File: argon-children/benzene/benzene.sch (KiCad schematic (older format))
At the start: 9 parts, among them U1 Conn1, U2 SPI FLASH, U3 Conn2

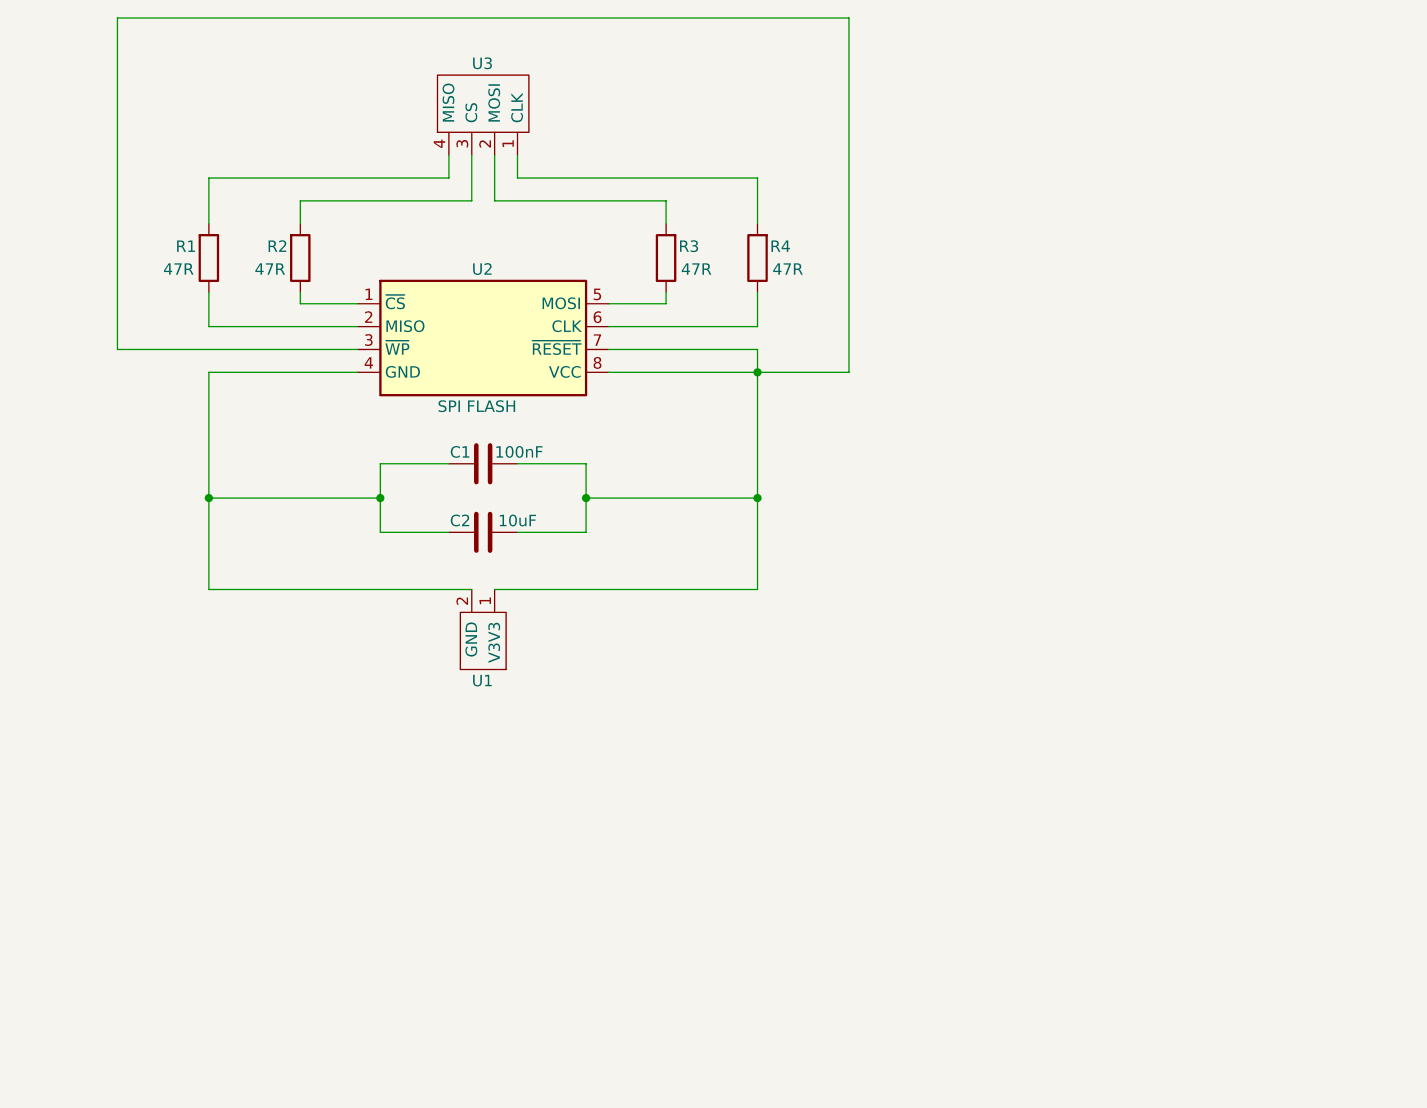
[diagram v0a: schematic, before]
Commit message: Add 555 to benzene
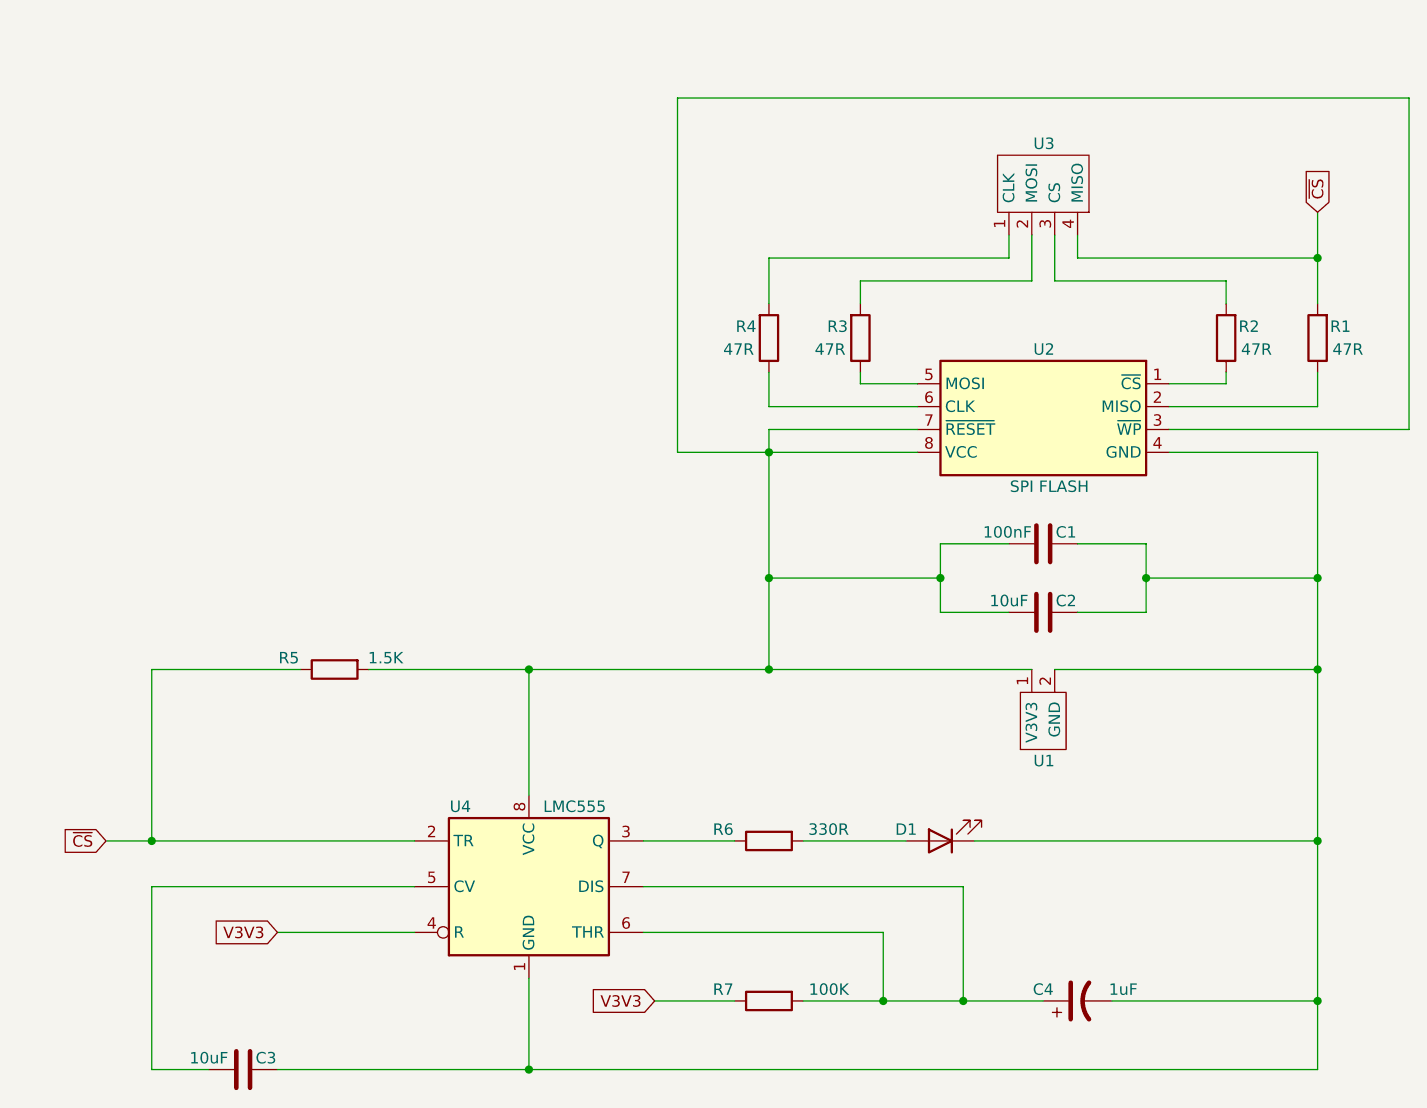
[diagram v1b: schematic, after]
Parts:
- added C3: 10uF, symbol Device:C
- added C4: 1uF, symbol Device:CP1
- added D1: LED, symbol Device:LED
- added R5: 1.5K, symbol Device:R
- added R6: 330R, symbol Device:R
- added R7: 100K, symbol Device:R
- added U4: LMC555, Package_SO:SOIC-8_3.9x4.9mm_P1.27mm, symbol Timer:LMC555xM
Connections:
- net at C1.1, C2.1, U1.1 (V3V3)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: now also R5.2, U4.8 (VCC)
- net at C1.2, C2.2, U1.2 (GND)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: now also C3.2, C4.2, D1.1 (K), U4.1 (GND)
- net ~CS: now reaches R1.2, U3.4 (MISO)
- net ~CS: now also R5.1, U4.2 (TR)
- new net: R6.1, U4.3 (Q)
- new net: C3.1, U4.5 (CV)
- new net: C4.1, R7.2, U4.6 (THR), U4.7 (DIS)
- new net: D1.2 (A), R6.2
- new net V3V3: R7.1, U4.4 (R)
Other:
- moved on the sheet: C1, C2, R1, R2, R3, R4, U1, U2, U3
